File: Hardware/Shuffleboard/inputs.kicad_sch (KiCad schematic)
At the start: 27 parts, among them U3 Comparator

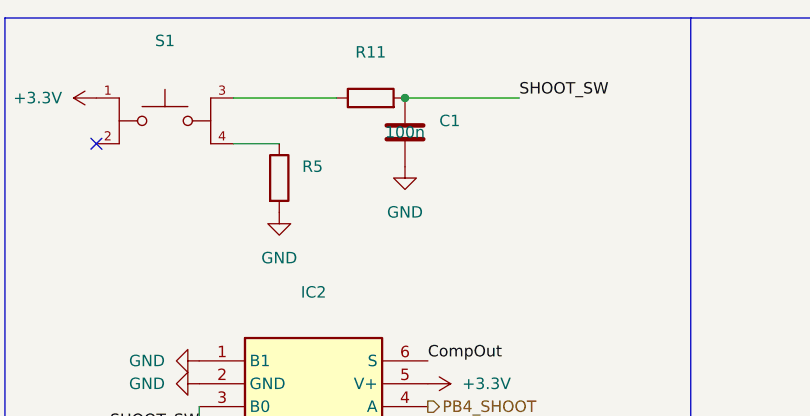
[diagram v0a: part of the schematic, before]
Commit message: updated to end
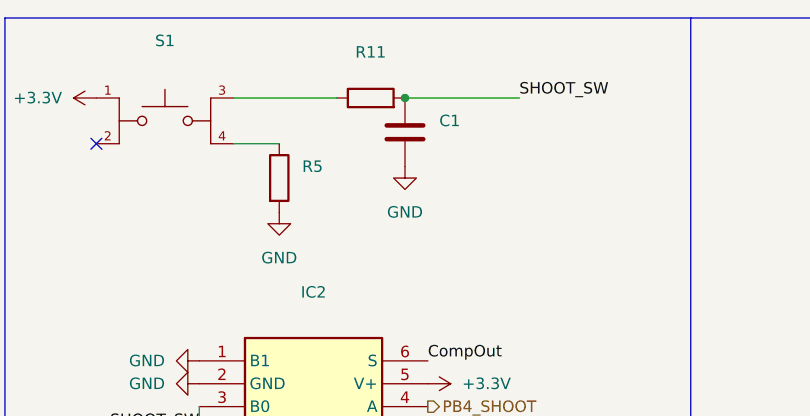
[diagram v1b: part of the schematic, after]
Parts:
- C1, C3, C4, C5, C7: value 100n -> (none)
- D1: value Red -> (none)
- R1, R12, R13, R45, R5, R9: value 10k -> (none)
- R10, R14: value 330 -> (none)
- R11, R2, R3, R4, R6: value 1k -> (none)
- U3: value Comparator -> (none)
